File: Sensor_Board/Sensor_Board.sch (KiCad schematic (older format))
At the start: 15 parts, among them J1 Mic_Conn, U1 TLV741PxxDQNx

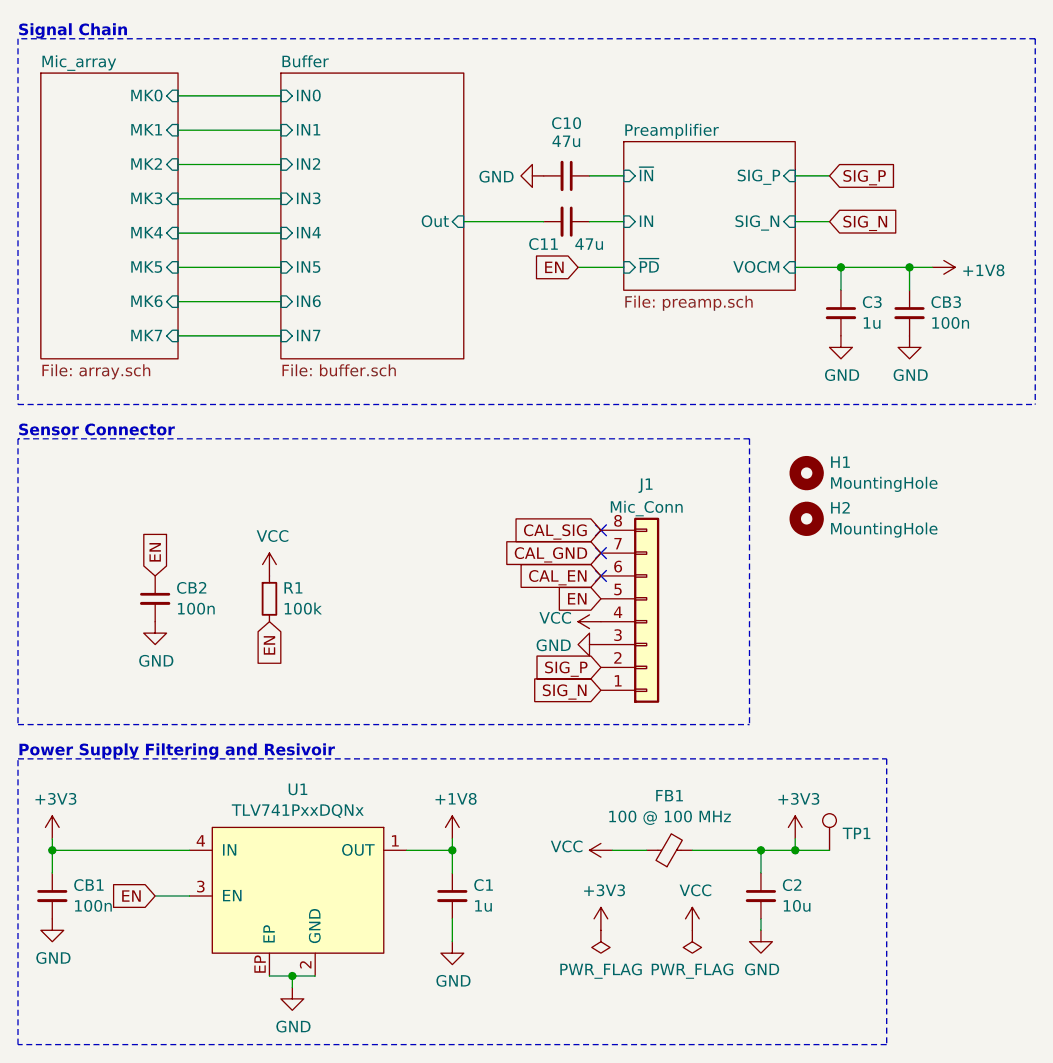
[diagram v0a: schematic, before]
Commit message: Start board layout
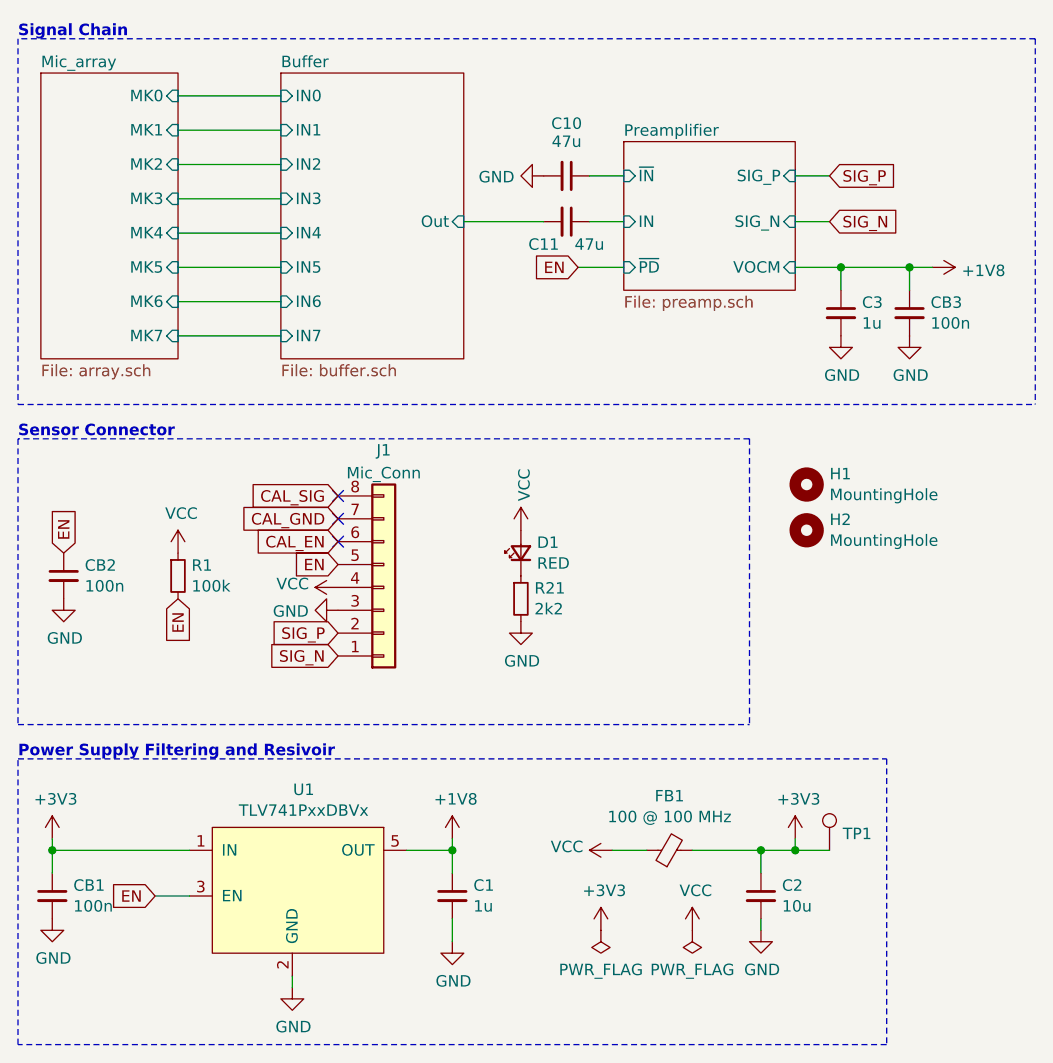
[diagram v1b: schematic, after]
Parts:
- removed U1: TLV741PxxDQNx, grootvoet:Texas_X2SON-4_1x1mm_P0.65mm, symbol grootvoet:TLV741PxxDQNx
- added D1: RED, LED_SMD:LED_0603_1608Metric_Pad1.05x0.95mm_HandSolder, symbol Device:LED_Small
- added R21: 2k2, Resistor_SMD:R_0603_1608Metric_Pad0.98x0.95mm_HandSolder, symbol Device:R_Small
- added U1: TLV741PxxDBVx, Package_TO_SOT_SMD:SOT-23-5, symbol grootvoet:TLV741PxxDBVx
- H1, H2: footprint MountingHole:MountingHole_2.7mm_M2.5_DIN965_Pad -> MountingHole:MountingHole_3.2mm_M3_Pad_Via
- J1: footprint Connector_PinHeader_2.54mm:PinHeader_1x08_P2.54mm_Vertical -> Connector_PinHeader_2.00mm:PinHeader_1x08_P2.00mm_Vertical
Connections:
- net +1V8: now also U1.5 (OUT)
- net +3V3: now also U1.1 (IN)
- net EN: now also U1.3 (EN)
- net GND: now also R21.2, U1.2 (GND)
- net VCC: now also D1.2 (A)
- new net: D1.1 (K), R21.1
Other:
- moved on the sheet: CB2, H1, H2, J1, R1
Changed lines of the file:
@@
 L Connector_Generic:Conn_01x08 J?
 U 1 1 5F9760C7
-P 5800 4200
+P 4650 4050
 AR Path="/5F1E182A/5F9760C7" Ref="J?"  Part="1"
 AR Path="/5EE5ECAD/5EE62C2B/5F9760C7" Ref="J?"  Part="1"
@@
 AR Path="/5F803BE9/5F9760C7" Ref="J?"  Part="1"
 AR Path="/5F9760C7" Ref="J1"  Part="1"
-F 0 "J1" H 5800 3600 50  0000 C CNN
-F 1 "Mic_Conn" H 5800 3700 50  0000 C CNN
-F 2 "Connector_PinHeader_2.54mm:PinHeader_1x08_P2.54mm_Vertical" H 5800 4200 50  0001 C CNN
-F 3 "~" H 5800 4200 50  0001 C CNN
-F 4 "" H 5800 4200 50  0001 C CNN "MPN"
-F 5 "" H 5800 4200 50  0001 C CNN "Mfr."
-	1    5800 4200
+F 0 "J1" H 4650 3450 50  0000 C CNN
+F 1 "Mic_Conn" H 4650 3550 50  0000 C CNN
+F 2 "Connector_PinHeader_2.00mm:PinHeader_1x08_P2.00mm_Vertical" H 4650 4050 50  0001 C CNN
+F 3 "~" H 4650 4050 50  0001 C CNN
+F 4 "" H 4650 4050 50  0001 C CNN "MPN"
+F 5 "" H 4650 4050 50  0001 C CNN "Mfr."
+	1    4650 4050
 	1    0    0    1
 $EndComp
@@
 L Device:R_Small R?
 U 1 1 5F976175
-P 4150 4100
+P 3750 4000
 AR Path="/5EE5ECAD/5EECE6B8/5F976175" Ref="R?"  Part="1"
 AR Path="/5EE5ECAD/5EF21991/5F976175" Ref="R?"  Part="1"
@@
 AR Path="/5F803BE9/5F976175" Ref="R?"  Part="1"
 AR Path="/5F976175" Ref="R1"  Part="1"
-F 0 "R1" H 4209 4146 50  0000 L CNN
-F 1 "100k" H 4209 4055 50  0000 L CNN
-F 2 "Resistor_SMD:R_0603_1608Metric_Pad0.98x0.95mm_HandSolder" H 4150 4100 50  0001 C CNN
-F 3 "~" H 4150 4100 50  0001 C CNN
-F 4 "RC0603FR-07100KL" H 4150 4100 50  0001 C CNN "MPN"
-F 5 "Yageo" H 4150 4100 50  0001 C CNN "Mfr."
-	1    4150 4100
+F 0 "R1" H 3809 4046 50  0000 L CNN
+F 1 "100k" H 3809 3955 50  0000 L CNN
+F 2 "Resistor_SMD:R_0603_1608Metric_Pad0.98x0.95mm_HandSolder" H 3750 4000 50  0001 C CNN
+F 3 "~" H 3750 4000 50  0001 C CNN
+F 4 "RC0603FR-07100KL" H 3750 4000 50  0001 C CNN "MPN"
+F 5 "Yageo" H 3750 4000 50  0001 C CNN "Mfr."
+	1    3750 4000
 	1    0    0    -1
 $EndComp
@@
 L Device:C_Small CB?
 U 1 1 5F976195
-P 3650 4100
+P 3250 4000
 AR Path="/5EE5ECAD/5EECE6B8/5F976195" Ref="CB?"  Part="1"
 AR Path="/5EE5ECAD/5EF21991/5F976195" Ref="CB?"  Part="1"
@@
 AR Path="/5F803BE9/5F976195" Ref="CB?"  Part="1"
 AR Path="/5F976195" Ref="CB2"  Part="1"
-F 0 "CB2" H 3742 4146 50  0000 L CNN
-F 1 "100n" H 3742 4055 50  0000 L CNN
-F 2 "Capacitor_SMD:C_0603_1608Metric_Pad1.08x0.95mm_HandSolder" H 3650 4100 50  0001 C CNN
-F 3 "~" H 3650 4100 50  0001 C CNN
-F 4 "C0603C104M5RACTU" H 3650 4100 50  0001 C CNN "MPN"
-F 5 "KEMET" H 3650 4100 50  0001 C CNN "Mfr."
-	1    3650 4100
+F 0 "CB2" H 3342 4046 50  0000 L CNN
+F 1 "100n" H 3342 3955 50  0000 L CNN
+F 2 "Capacitor_SMD:C_0603_1608Metric_Pad1.08x0.95mm_HandSolder" H 3250 4000 50  0001 C CNN
+F 3 "~" H 3250 4000 50  0001 C CNN
+F 4 "C0603C104M5RACTU" H 3250 4000 50  0001 C CNN "MPN"
+F 5 "KEMET" H 3250 4000 50  0001 C CNN "Mfr."
+	1    3250 4000
 	1    0    0    -1
 $EndComp
@@
 L Mechanical:MountingHole H?
 U 1 1 5F9761A0
-P 6500 3750
+P 6500 3800
 AR Path="/5EE5ECAD/5EECE6B8/5F9761A0" Ref="H?"  Part="1"
 AR Path="/5EE5ECAD/5EF4C631/5F9761A0" Ref="H?"  Part="1"
@@
 AR Path="/5F803BE9/5F9761A0" Ref="H?"  Part="1"
 AR Path="/5F9761A0" Ref="H2"  Part="1"
-F 0 "H2" H 6600 3796 50  0000 L CNN
-F 1 "MountingHole" H 6600 3705 50  0000 L CNN
-F 2 "MountingHole:MountingHole_2.7mm_M2.5_DIN965_Pad" H 6500 3750 50  0001 C CNN
-F 3 "~" H 6500 3750 50  0001 C CNN
-	1    6500 3750
+F 0 "H2" H 6600 3846 50  0000 L CNN
+F 1 "MountingHole" H 6600 3755 50  0000 L CNN
+F 2 "MountingHole:MountingHole_3.2mm_M3_Pad_Via" H 6500 3800 50  0001 C CNN
+F 3 "~" H 6500 3800 50  0001 C CNN
+	1    6500 3800
 	1    0    0    -1
 $EndComp
@@
 L Mechanical:MountingHole H?
 U 1 1 5F9761A6
-P 6500 3550
+P 6500 3600
 AR Path="/5EE5ECAD/5EECE6B8/5F9761A6" Ref="H?"  Part="1"
 AR Path="/5EE5ECAD/5EF4C631/5F9761A6" Ref="H?"  Part="1"
@@
 AR Path="/5F803BE9/5F9761A6" Ref="H?"  Part="1"
 AR Path="/5F9761A6" Ref="H1"  Part="1"
-F 0 "H1" H 6600 3596 50  0000 L CNN
-F 1 "MountingHole" H 6600 3505 50  0000 L CNN
-F 2 "MountingHole:MountingHole_2.7mm_M2.5_DIN965_Pad" H 6500 3550 50  0001 C CNN
-F 3 "~" H 6500 3550 50  0001 C CNN
-	1    6500 3550
+F 0 "H1" H 6600 3646 50  0000 L CNN
+F 1 "MountingHole" H 6600 3555 50  0000 L CNN
+F 2 "MountingHole:MountingHole_3.2mm_M3_Pad_Via" H 6500 3600 50  0001 C CNN
+F 3 "~" H 6500 3600 50  0001 C CNN
+	1    6500 3600
 	1    0    0    -1
 $EndComp
@@
 F 5 "KEMET" H 6300 5400 50  0001 C CNN "Mfr."
 	1    6300 5400
-	1    0    0    -1
-$EndComp
-$Comp
-L grootvoet:TLV741PxxDQNx U1
-U 1 1 5F9A84F9
-P 4250 5300
-F 0 "U1" H 4275 5665 50  0000 C CNN
-F 1 "TLV741PxxDQNx" H 4275 5574 50  0000 C CNN
-F 2 "grootvoet:Texas_X2SON-4_1x1mm_P0.65mm" H 4650 4900 50  0001 C CNN
-F 3 "" H 4650 4900 50  0001 C CNN
-F 4 "TLV74118PDQNR" H 4250 5300 50  0001 C CNN "MFN"
-F 5 "TI" H 4250 5300 50  0001 C CNN "Mfr."
-	1    4250 5300
 	1    0    0    -1
 $EndComp
@@
 Wire Wire Line
 	4250 5800 4250 5750
-Wire Wire Line
-	4250 5750 4350 5750
-Wire Wire Line
-	4250 5750 4150 5750
-Connection ~ 4250 5750
-Text GLabel 5600 3800 0    50   Input ~ 0
+Text GLabel 4450 3650 0    50   Input ~ 0
 CAL_SIG
-Text GLabel 5600 3900 0    50   Input ~ 0
+Text GLabel 4450 3750 0    50   Input ~ 0
 CAL_GND
-Text GLabel 5600 4000 0    50   Input ~ 0
+Text GLabel 4450 3850 0    50   Input ~ 0
 CAL_EN
-Text GLabel 5600 4100 0    50   Input ~ 0
+Text GLabel 4450 3950 0    50   Input ~ 0
 EN
-Text GLabel 5600 4400 0    50   Input ~ 0
+Text GLabel 4450 4250 0    50   Input ~ 0
 SIG_P
-Text GLabel 5600 4500 0    50   Input ~ 0
+Text GLabel 4450 4350 0    50   Input ~ 0
 SIG_N
 $Comp
 L power:VCC #PWR09
 U 1 1 5FA24F87
-P 5600 4200
-F 0 "#PWR09" H 5600 4050 50  0001 C CNN
-F 1 "VCC" V 5615 4327 50  0000 L CNN
-F 2 "" H 5600 4200 50  0001 C CNN
-F 3 "" H 5600 4200 50  0001 C CNN
-	1    5600 4200
+P 4450 4050
+F 0 "#PWR09" H 4450 3900 50  0001 C CNN
+F 1 "VCC" V 4465 4177 50  0000 L CNN
+F 2 "" H 4450 4050 50  0001 C CNN
+F 3 "" H 4450 4050 50  0001 C CNN
+	1    4450 4050
 	0    -1   -1   0
 $EndComp
@@
 L power:GND #PWR010
 U 1 1 5FA257DC
-P 5600 4300
-F 0 "#PWR010" H 5600 4050 50  0001 C CNN
-F 1 "GND" V 5605 4172 50  0000 R CNN
-F 2 "" H 5600 4300 50  0001 C CNN
-F 3 "" H 5600 4300 50  0001 C CNN
-	1    5600 4300
+P 4450 4150
+F 0 "#PWR010" H 4450 3900 50  0001 C CNN
+F 1 "GND" V 4455 4022 50  0000 R CNN
+F 2 "" H 4450 4150 50  0001 C CNN
+F 3 "" H 4450 4150 50  0001 C CNN
+	1    4450 4150
 	0    1    1    0
 $EndComp
@@
 L power:GND #PWR03
 U 1 1 5FA272C8
-P 3650 4200
-F 0 "#PWR03" H 3650 3950 50  0001 C CNN
-F 1 "GND" H 3655 4027 50  0000 C CNN
-F 2 "" H 3650 4200 50  0001 C CNN
-F 3 "" H 3650 4200 50  0001 C CNN
-	1    3650 4200
-	1    0    0    -1
-$EndComp
-Text GLabel 3650 4000 1    50   Input ~ 0
+P 3250 4100
+F 0 "#PWR03" H 3250 3850 50  0001 C CNN
+F 1 "GND" H 3255 3927 50  0000 C CNN
+F 2 "" H 3250 4100 50  0001 C CNN
+F 3 "" H 3250 4100 50  0001 C CNN
+	1    3250 4100
+	1    0    0    -1
+$EndComp
+Text GLabel 3250 3900 1    50   Input ~ 0
 EN
-Text GLabel 4150 4200 3    50   Input ~ 0
+Text GLabel 3750 4100 3    50   Input ~ 0
 EN
 $Comp
@@
 L power:VCC #PWR04
 U 1 1 5FA6370F
-P 4150 4000
-F 0 "#PWR04" H 4150 3850 50  0001 C CNN
-F 1 "VCC" H 4165 4173 50  0000 C CNN
-F 2 "" H 4150 4000 50  0001 C CNN
-F 3 "" H 4150 4000 50  0001 C CNN
-	1    4150 4000
+P 3750 3900
+F 0 "#PWR04" H 3750 3750 50  0001 C CNN
+F 1 "VCC" H 3765 4073 50  0000 C CNN
+F 2 "" H 3750 3900 50  0001 C CNN
+F 3 "" H 3750 3900 50  0001 C CNN
+	1    3750 3900
 	1    0    0    -1
 $EndComp
@@
 Text Notes 3050 1650 0    50   ~ 10
 Signal Chain
-NoConn ~ 5600 4000
-NoConn ~ 5600 3900
-NoConn ~ 5600 3800
+NoConn ~ 4450 3850
+NoConn ~ 4450 3750
+NoConn ~ 4450 3650
 $Comp
 L power:+3V3 #PWR01
@@
 Wire Wire Line
 	5350 2450 5000 2450
+$Comp
+L grootvoet:TLV741PxxDBVx U1
+U 1 1 5F90B83C
+P 4250 5300
+F 0 "U1" H 4300 5665 50  0000 C CNN
+F 1 "TLV741PxxDBVx" H 4300 5574 50  0000 C CNN
+F 2 "Package_TO_SOT_SMD:SOT-23-5" H 4650 4900 50  0001 C CNN
+F 3 "" H 4650 4900 50  0001 C CNN
+	1    4250 5300
+	1    0    0    -1
+$EndComp
+$Comp
+L Device:LED_Small D1
+U 1 1 5F915892
+P 5250 3900
+F 0 "D1" V 5296 3830 50  0000 R CNN
+F 1 "RED" V 5205 3830 50  0000 R CNN
+F 2 "LED_SMD:LED_0603_1608Metric_Pad1.05x0.95mm_HandSolder" V 5250 3900 50  0001 C CNN
+F 3 "~" V 5250 3900 50  0001 C CNN
+	1    5250 3900
+	0    -1   -1   0
+$EndComp
+$Comp
+L Device:R_Small R?
+U 1 1 5F915C70
+P 5250 4100
+AR Path="/5EE5ECAD/5EECE6B8/5F915C70" Ref="R?"  Part="1"
+AR Path="/5EE5ECAD/5EF21991/5F915C70" Ref="R?"  Part="1"
+AR Path="/5EE5ECAD/5EF33EA2/5F915C70" Ref="R?"  Part="1"
+AR Path="/5EE5ECAD/5EF4C631/5F915C70" Ref="R?"  Part="1"
+AR Path="/5EE5ECAD/5F0013E5/5F915C70" Ref="R?"  Part="1"
+AR Path="/5EE5ECAD/5F0090C7/5F915C70" Ref="R?"  Part="1"
+AR Path="/5F803BE9/5F915C70" Ref="R?"  Part="1"
+AR Path="/5F915C70" Ref="R21"  Part="1"
+F 0 "R21" H 5309 4146 50  0000 L CNN
+F 1 "2k2" H 5309 4055 50  0000 L CNN
+F 2 "Resistor_SMD:R_0603_1608Metric_Pad0.98x0.95mm_HandSolder" H 5250 4100 50  0001 C CNN
+F 3 "~" H 5250 4100 50  0001 C CNN
+F 4 "" H 5250 4100 50  0001 C CNN "MPN"
+F 5 "Yageo" H 5250 4100 50  0001 C CNN "Mfr."
+	1    5250 4100
+	1    0    0    -1
+$EndComp
+$Comp
+L power:GND #PWR064
+U 1 1 5F91626C
+P 5250 4200
+F 0 "#PWR064" H 5250 3950 50  0001 C CNN
+F 1 "GND" H 5255 4027 50  0000 C CNN
+F 2 "" H 5250 4200 50  0001 C CNN
+F 3 "" H 5250 4200 50  0001 C CNN
+	1    5250 4200
+	1    0    0    -1
+$EndComp
+$Comp
+L power:VCC #PWR063
+U 1 1 5F9167F7
+P 5250 3800
+F 0 "#PWR063" H 5250 3650 50  0001 C CNN
+F 1 "VCC" V 5265 3927 50  0000 L CNN
+F 2 "" H 5250 3800 50  0001 C CNN
+F 3 "" H 5250 3800 50  0001 C CNN
+	1    5250 3800
+	1    0    0    -1
+$EndComp
 $EndSCHEMATC

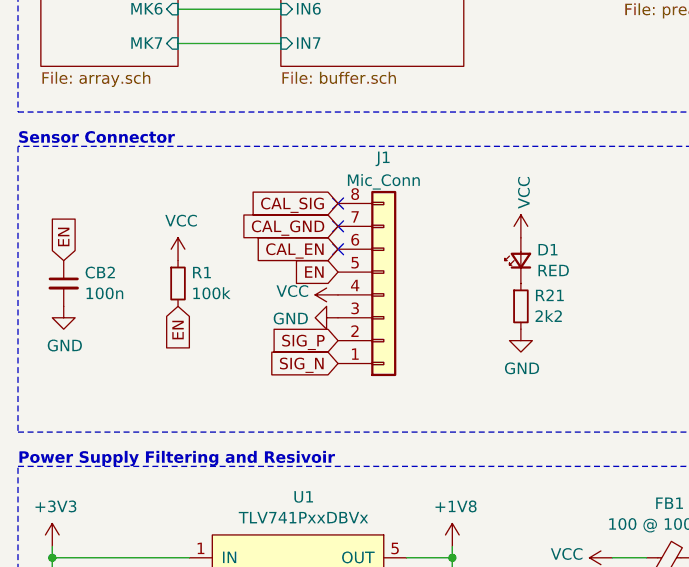
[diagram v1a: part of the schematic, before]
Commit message: Add connector
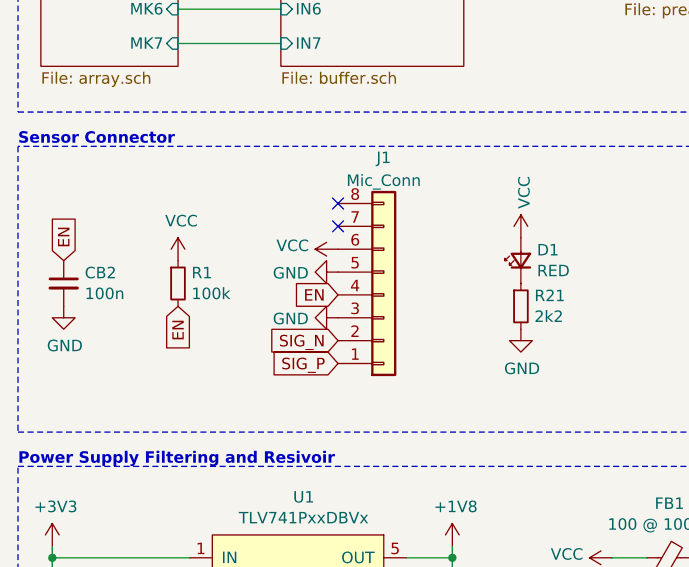
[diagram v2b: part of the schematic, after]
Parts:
- J1: footprint Connector_PinHeader_2.00mm:PinHeader_1x08_P2.00mm_Vertical -> grootvoet:TE_7-215079-8; MPN (none) -> 7-215079-8, 7-215083-8; Mfr. (none) -> TE Connectivity
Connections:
- net CAL_EN is gone; now on net VCC: J1.6 (Pin_6)
- net EN: now also J1.4 (Pin_4); no longer J1.5 (Pin_5)
- net GND: now also J1.5 (Pin_5)
- net SIG_N: now also J1.2 (Pin_2); no longer J1.1 (Pin_1)
- net SIG_P: now also J1.1 (Pin_1); no longer J1.2 (Pin_2)
- net VCC: no longer J1.4 (Pin_4)
- net CAL_GND: no longer names the net of J1.7 (Pin_7)
- net CAL_SIG: no longer names the net of J1.8 (Pin_8)
- no-connect marks 3 -> 2
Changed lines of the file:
@@
 Comment4 "CM Geldenhuys"
 $EndDescr
-$Comp
-L Connector_Generic:Conn_01x08 J?
-U 1 1 5F9760C7
-P 4650 4050
-AR Path="/5F1E182A/5F9760C7" Ref="J?"  Part="1"
-AR Path="/5EE5ECAD/5EE62C2B/5F9760C7" Ref="J?"  Part="1"
-AR Path="/5EE5ECAD/5EE62C39/5F9760C7" Ref="J?"  Part="1"
-AR Path="/5EE5ECAD/5EE62C47/5F9760C7" Ref="J?"  Part="1"
-AR Path="/5EE5ECAD/5EE62C55/5F9760C7" Ref="J?"  Part="1"
-AR Path="/5EE5ECAD/5EE8F49C/5F9760C7" Ref="J?"  Part="1"
-AR Path="/5EE5ECAD/5EE91C9A/5F9760C7" Ref="J?"  Part="1"
-AR Path="/5EE5ECAD/5EE94935/5F9760C7" Ref="J?"  Part="1"
-AR Path="/5EE1D522/5F9760C7" Ref="J?"  Part="1"
-AR Path="/5EE5ECAD/5EECE6B8/5F9760C7" Ref="J?"  Part="1"
-AR Path="/5EE5ECAD/5EF21991/5F9760C7" Ref="J?"  Part="1"
-AR Path="/5EE5ECAD/5EF33EA2/5F9760C7" Ref="J?"  Part="1"
-AR Path="/5EE5ECAD/5EF4C631/5F9760C7" Ref="J?"  Part="1"
-AR Path="/5EE5ECAD/5F0013E5/5F9760C7" Ref="J?"  Part="1"
-AR Path="/5EE5ECAD/5F0090C7/5F9760C7" Ref="J?"  Part="1"
-AR Path="/5F803BE9/5F9760C7" Ref="J?"  Part="1"
-AR Path="/5F9760C7" Ref="J1"  Part="1"
-F 0 "J1" H 4650 3450 50  0000 C CNN
-F 1 "Mic_Conn" H 4650 3550 50  0000 C CNN
-F 2 "Connector_PinHeader_2.00mm:PinHeader_1x08_P2.00mm_Vertical" H 4650 4050 50  0001 C CNN
-F 3 "~" H 4650 4050 50  0001 C CNN
-F 4 "" H 4650 4050 50  0001 C CNN "MPN"
-F 5 "" H 4650 4050 50  0001 C CNN "Mfr."
-	1    4650 4050
-	1    0    0    1
-$EndComp
 Text Notes 3050 4800 0    50   ~ 10
 Power Supply Filtering and Resivoir
@@
 Wire Wire Line
 	4250 5800 4250 5750
-Text GLabel 4450 3650 0    50   Input ~ 0
-CAL_SIG
-Text GLabel 4450 3750 0    50   Input ~ 0
-CAL_GND
-Text GLabel 4450 3850 0    50   Input ~ 0
-CAL_EN
-Text GLabel 4450 3950 0    50   Input ~ 0
+Text GLabel 4450 4050 0    50   Input ~ 0
 EN
-Text GLabel 4450 4250 0    50   Input ~ 0
-SIG_P
-Text GLabel 4450 4350 0    50   Input ~ 0
-SIG_N
 $Comp
 L power:VCC #PWR09
 U 1 1 5FA24F87
-P 4450 4050
-F 0 "#PWR09" H 4450 3900 50  0001 C CNN
-F 1 "VCC" V 4465 4177 50  0000 L CNN
-F 2 "" H 4450 4050 50  0001 C CNN
-F 3 "" H 4450 4050 50  0001 C CNN
-	1    4450 4050
+P 4450 3850
+F 0 "#PWR09" H 4450 3700 50  0001 C CNN
+F 1 "VCC" V 4465 3977 50  0000 L CNN
+F 2 "" H 4450 3850 50  0001 C CNN
+F 3 "" H 4450 3850 50  0001 C CNN
+	1    4450 3850
 	0    -1   -1   0
 $EndComp
@@
 Text Notes 3050 1650 0    50   ~ 10
 Signal Chain
-NoConn ~ 4450 3850
 NoConn ~ 4450 3750
 NoConn ~ 4450 3650
@@
 	1    0    0    -1
 $EndComp
+$Comp
+L Connector_Generic:Conn_01x08 J?
+U 1 1 5F9760C7
+P 4650 4050
+AR Path="/5F1E182A/5F9760C7" Ref="J?"  Part="1"
+AR Path="/5EE5ECAD/5EE62C2B/5F9760C7" Ref="J?"  Part="1"
+AR Path="/5EE5ECAD/5EE62C39/5F9760C7" Ref="J?"  Part="1"
+AR Path="/5EE5ECAD/5EE62C47/5F9760C7" Ref="J?"  Part="1"
+AR Path="/5EE5ECAD/5EE62C55/5F9760C7" Ref="J?"  Part="1"
+AR Path="/5EE5ECAD/5EE8F49C/5F9760C7" Ref="J?"  Part="1"
+AR Path="/5EE5ECAD/5EE91C9A/5F9760C7" Ref="J?"  Part="1"
+AR Path="/5EE5ECAD/5EE94935/5F9760C7" Ref="J?"  Part="1"
+AR Path="/5EE1D522/5F9760C7" Ref="J?"  Part="1"
+AR Path="/5EE5ECAD/5EECE6B8/5F9760C7" Ref="J?"  Part="1"
+AR Path="/5EE5ECAD/5EF21991/5F9760C7" Ref="J?"  Part="1"
+AR Path="/5EE5ECAD/5EF33EA2/5F9760C7" Ref="J?"  Part="1"
+AR Path="/5EE5ECAD/5EF4C631/5F9760C7" Ref="J?"  Part="1"
+AR Path="/5EE5ECAD/5F0013E5/5F9760C7" Ref="J?"  Part="1"
+AR Path="/5EE5ECAD/5F0090C7/5F9760C7" Ref="J?"  Part="1"
+AR Path="/5F803BE9/5F9760C7" Ref="J?"  Part="1"
+AR Path="/5F9760C7" Ref="J1"  Part="1"
+F 0 "J1" H 4650 3450 50  0000 C CNN
+F 1 "Mic_Conn" H 4650 3550 50  0000 C CNN
+F 2 "grootvoet:TE_7-215079-8" H 4650 4050 50  0001 C CNN
+F 3 "~" H 4650 4050 50  0001 C CNN
+F 4 "7-215079-8, 7-215083-8" H 4650 4050 50  0001 C CNN "MPN"
+F 5 "TE Connectivity" H 4650 4050 50  0001 C CNN "Mfr."
+	1    4650 4050
+	1    0    0    1
+$EndComp
+$Comp
+L power:GND #PWR0101
+U 1 1 5F8DD1D1
+P 4450 3950
+F 0 "#PWR0101" H 4450 3700 50  0001 C CNN
+F 1 "GND" V 4455 3822 50  0000 R CNN
+F 2 "" H 4450 3950 50  0001 C CNN
+F 3 "" H 4450 3950 50  0001 C CNN
+	1    4450 3950
+	0    1    1    0
+$EndComp
+Text GLabel 4450 4350 0    50   Input ~ 0
+SIG_P
+Text GLabel 4450 4250 0    50   Input ~ 0
+SIG_N
 $EndSCHEMATC
